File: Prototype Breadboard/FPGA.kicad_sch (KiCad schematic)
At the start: 1 part, among them U3 XC7Z010-1CLG225I

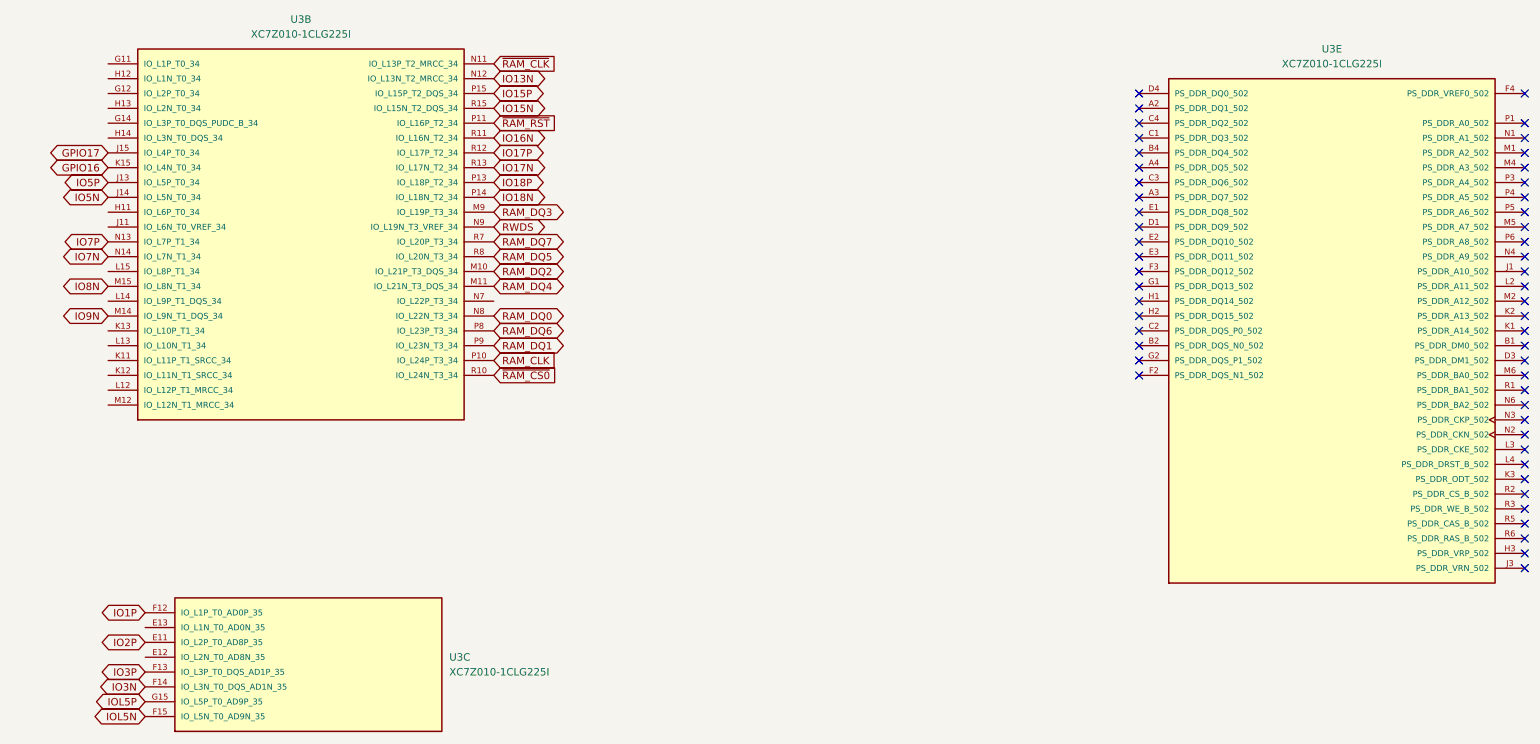
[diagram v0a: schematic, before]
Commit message: 1/4 update
update the breadboard version
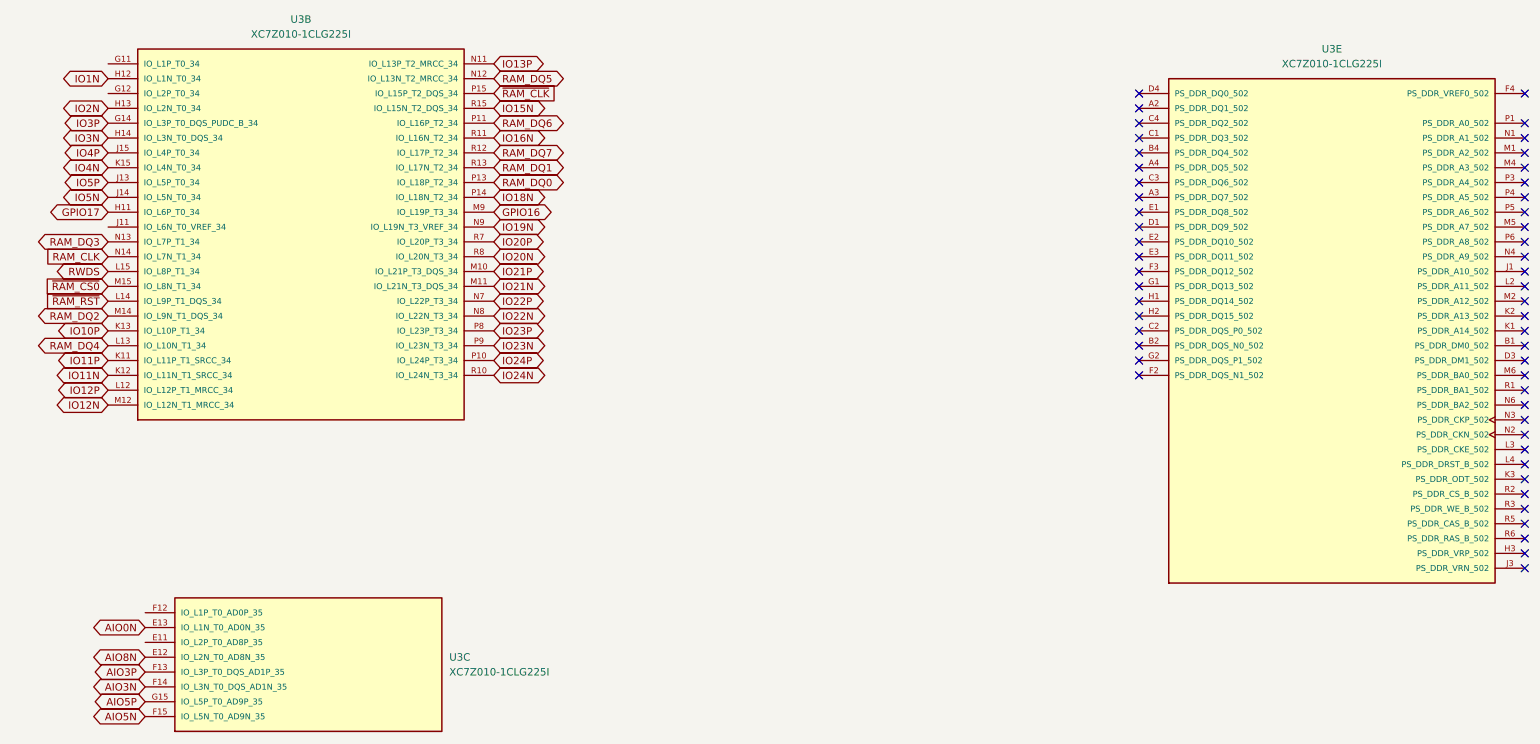
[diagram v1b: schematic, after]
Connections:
- net IO13N is gone; now on net RAM_DQ5: U3.N12 (IO_L13N_T2_MRCC_34)
- net IO15P is gone; now on net ~{RAM_CLK}: U3.P15 (IO_L15P_T2_DQS_34)
- net IO17N is gone; now on net RAM_DQ1: U3.R13 (IO_L17N_T2_34)
- net IO17P is gone; now on net RAM_DQ7: U3.R12 (IO_L17P_T2_34)
- net IO18P is gone; now on net RAM_DQ0: U3.P13 (IO_L18P_T2_34)
- net IO7N is gone; now on net RAM_CLK: U3.N14 (IO_L7N_T1_34)
- net IO7P is gone; now on net RAM_DQ3: U3.N13 (IO_L7P_T1_34)
- net IO8N is gone; now on net ~{RAM_CS0}: U3.M15 (IO_L8N_T1_34)
- net IO9N is gone; now on net RAM_DQ2: U3.M14 (IO_L9N_T1_DQS_34)
- net GPIO16: now also U3.M9 (IO_L19P_T3_34); no longer U3.K15 (IO_L4N_T0_34)
- net GPIO17: now also U3.H11 (IO_L6P_T0_34); no longer U3.J15 (IO_L4P_T0_34)
- net IO3N: now also U3.H14 (IO_L3N_T0_DQS_34); no longer U3.F14 (IO_L3N_T0_DQS_AD1N_35)
- net IO3P: now also U3.G14 (IO_L3P_T0_DQS_PUDC_B_34); no longer U3.F13 (IO_L3P_T0_DQS_AD1P_35)
- net RAM_CLK: no longer U3.P10 (IO_L24P_T3_34)
- net RAM_DQ0: no longer U3.N8 (IO_L22N_T3_34)
- net RAM_DQ1: no longer U3.P9 (IO_L23N_T3_34)
- net RAM_DQ2: no longer U3.M10 (IO_L21P_T3_DQS_34)
- net RAM_DQ3: no longer U3.M9 (IO_L19P_T3_34)
- net RAM_DQ4: now also U3.L13 (IO_L10N_T1_34); no longer U3.M11 (IO_L21N_T3_DQS_34)
- net RAM_DQ5: no longer U3.R8 (IO_L20N_T3_34)
- net RAM_DQ6: now also U3.P11 (IO_L16P_T2_34); no longer U3.P8 (IO_L23P_T3_34)
- net RAM_DQ7: no longer U3.R7 (IO_L20P_T3_34)
- net RWDS: now also U3.L15 (IO_L8P_T1_34); no longer U3.N9 (IO_L19N_T3_VREF_34)
- net ~{RAM_CLK}: no longer U3.N11 (IO_L13P_T2_MRCC_34)
- net ~{RAM_CS0}: no longer U3.R10 (IO_L24N_T3_34)
- net ~{RAM_RST}: now also U3.L14 (IO_L9P_T1_DQS_34); no longer U3.P11 (IO_L16P_T2_34)
- net IO1N: now reaches U3.H12 (IO_L1N_T0_34)
- net IO2N: now reaches U3.H13 (IO_L2N_T0_34)
- net IO11P: now reaches U3.K11 (IO_L11P_T1_SRCC_34)
- net IO11N: now reaches U3.K12 (IO_L11N_T1_SRCC_34)
- net IO10P: now reaches U3.K13 (IO_L10P_T1_34)
- net IO12P: now reaches U3.L12 (IO_L12P_T1_MRCC_34)
- net IO12N: now reaches U3.M12 (IO_L12N_T1_MRCC_34)
- net IO22P: now reaches U3.N7 (IO_L22P_T3_34)
- net AIO8N: now reaches U3.E12 (IO_L2N_T0_AD8N_35)
- net AIO0N: now reaches U3.E13 (IO_L1N_T0_AD0N_35)
- net IO1P: no longer names the net of U3.F12 (IO_L1P_T0_AD0P_35)
- net IO2P: no longer names the net of U3.E11 (IO_L2P_T0_AD8P_35)
- net IOL5N renamed AIO5N
- net IOL5P renamed AIO5P
- new net AIO3N: U3.F14 (IO_L3N_T0_DQS_AD1N_35)
- new net AIO3P: U3.F13 (IO_L3P_T0_DQS_AD1P_35)
- new net IO13P: U3.N11 (IO_L13P_T2_MRCC_34)
- new net IO19N: U3.N9 (IO_L19N_T3_VREF_34)
- new net IO20N: U3.R8 (IO_L20N_T3_34)
- new net IO20P: U3.R7 (IO_L20P_T3_34)
- new net IO21N: U3.M11 (IO_L21N_T3_DQS_34)
- new net IO21P: U3.M10 (IO_L21P_T3_DQS_34)
- new net IO22N: U3.N8 (IO_L22N_T3_34)
- new net IO23N: U3.P9 (IO_L23N_T3_34)
- new net IO23P: U3.P8 (IO_L23P_T3_34)
- new net IO24N: U3.R10 (IO_L24N_T3_34)
- new net IO24P: U3.P10 (IO_L24P_T3_34)
- new net IO4N: U3.K15 (IO_L4N_T0_34)
- new net IO4P: U3.J15 (IO_L4P_T0_34)
